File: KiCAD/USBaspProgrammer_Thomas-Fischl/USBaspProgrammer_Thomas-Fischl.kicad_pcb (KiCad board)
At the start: 2 copper layers, 73.7 x 31.8 mm, 22 parts, among them J1 USB_B, J2 ISP_header_Conn_02x05_Odd_Even, U1 ATmega88-20PU, Y1 12MHz

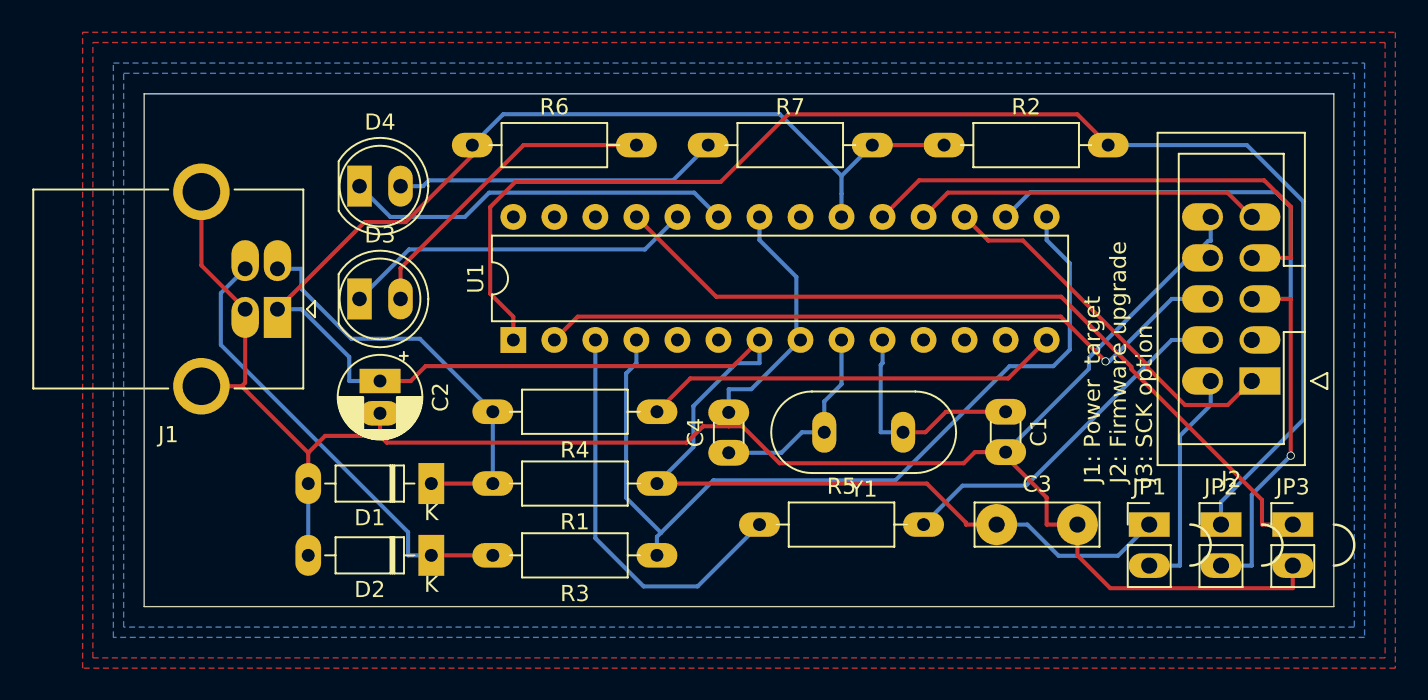
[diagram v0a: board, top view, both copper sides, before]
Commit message: kicad
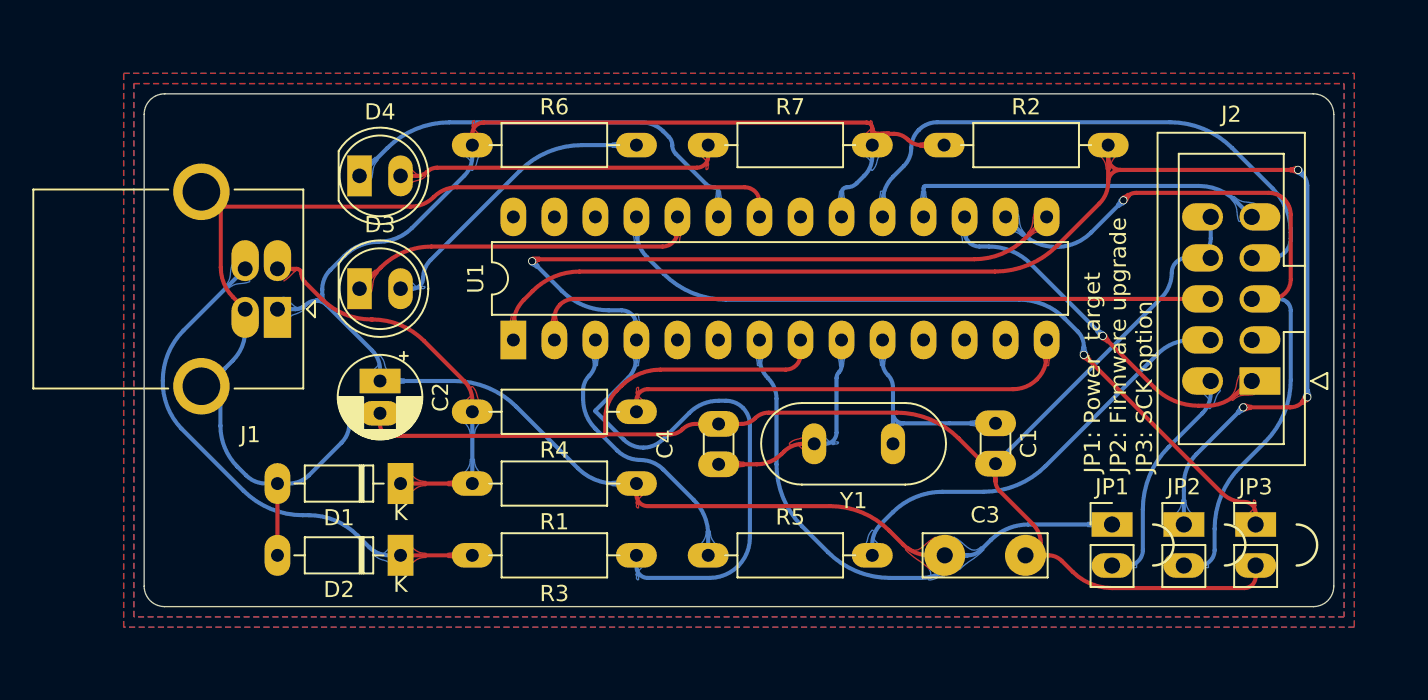
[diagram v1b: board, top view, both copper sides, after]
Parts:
- U1: footprint Package_DIP:DIP-28_W7.62mm -> My_Misc:DIP-28_W7.62mm_LongPads w socket
- moved C3 3.74 mm to (164.5, 125.7)
- moved R5 3.70 mm to (149.9, 125.7)
- moved JP2 2.30 mm to (179.3, 123.8)
- moved JP3 2.30 mm to (183.8, 123.8)
- moved JP1 2.30 mm to (174.9, 123.8)
- moved D1 1.91 mm to (130.8, 121.3)
- moved D2 1.91 mm to (130.8, 125.7)
- moved R1 1.27 mm to (145.4, 121.3)
- moved R3 1.27 mm to (145.4, 125.7)
- moved R4 1.27 mm to (145.4, 116.8)
- moved C1 0.95 mm to (167.7, 117.6)
- moved Y1 0.95 mm to (161.3, 118.8)
- moved C4 0.95 mm to (150.5, 120.1)
- moved D3 0.64 mm to (128.3, 109.2)
- moved D4 0.64 mm to (128.3, 102.2)
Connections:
- J2 pad 3: Net-(J2-Pad3) -> unconnected-(J2-Pad3)
- U1 pad 11: Net-(U1-Pad11) -> unconnected-(U1-Pad11)
- U1 pad 12: Net-(U1-Pad12) -> unconnected-(U1-Pad12)
- U1 pad 13: Net-(U1-Pad13) -> unconnected-(U1-Pad13)
- U1 pad 21: Net-(U1-Pad21) -> unconnected-(U1-Pad21)
- U1 pad 26: Net-(U1-Pad26) -> unconnected-(U1-Pad26)
- U1 pad 27: Net-(U1-Pad27) -> unconnected-(U1-Pad27)
- U1 pad 28: Net-(U1-Pad28) -> unconnected-(U1-Pad28)
- U1 pad 5: Net-(U1-Pad5) -> unconnected-(U1-Pad5)
- U1 pad 6: Net-(U1-Pad6) -> unconnected-(U1-Pad6)
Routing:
- net GND: track 137.7 -> 174.5 mm
- net Net-(R3-Pad1): track 53.4 -> 75.8 mm, vias 0 -> 1
- net Net-(R5-Pad1): track 25.3 -> 17.3 mm
- net +5V: track 130.7 -> 136.5 mm
- net Net-(D2-Pad1): track 28.4 -> 32.8 mm
- net Net-(J2-Pad4): track 22.5 -> 26.6 mm
- net Net-(J2-Pad7): track 32.5 -> 35.9 mm
- net Net-(R4-Pad1): track 26.0 -> 28.6 mm
- net RedLED: track 24.3 -> 26.9 mm
- net Net-(JP3-Pad1): track 49.5 -> 47.7 mm, vias 0 -> 1
- net Net-(JP2-Pad1): track 85.9 -> 84.5 mm, vias 0 -> 3
- net Net-(J2-Pad6): track 44.0 -> 42.7 mm, vias 1 -> 0
- net Net-(D3-Pad2): track 19.7 -> 18.4 mm
- net Net-(J2-Pad9): track 21.6 -> 22.8 mm
- net XTAL1: track 12.6 -> 13.8 mm
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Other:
- outline, holes or cut-outs redrawn
- board text added: "JP1: Power target JP2: Firmware upgrade JP3: SCK option"
- board text removed: "J1: Power target J2: Firmware upgrade J3: SCK option"
